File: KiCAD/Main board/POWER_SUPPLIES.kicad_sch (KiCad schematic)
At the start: 1 part, among them U18 12V

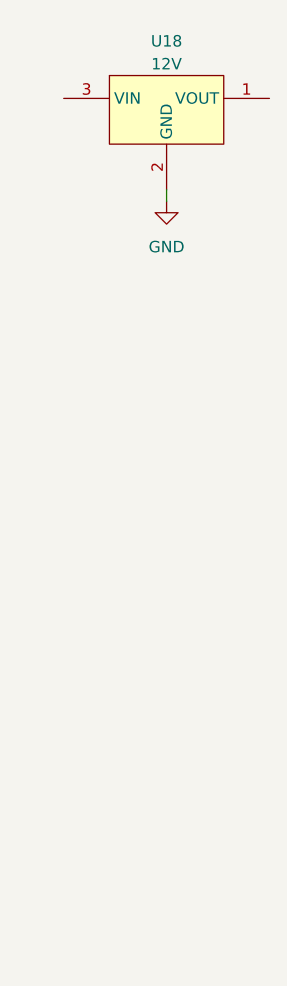
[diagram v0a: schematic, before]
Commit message: Worked on KiCAD
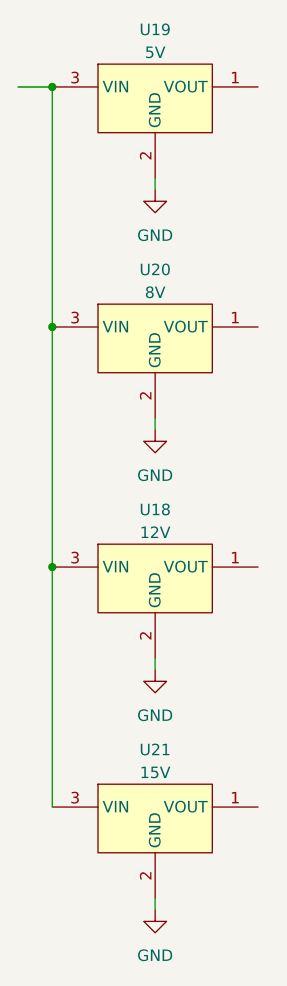
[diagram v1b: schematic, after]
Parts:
- added U19: 5V, Audio-DSP:BUCK_MAX17634C, symbol Audio_DSP:BUCK_5V_MAX17634C
- added U20: 8V, Audio-DSP:BUCK_MAX17634C, symbol Audio_DSP:BUCK_8V_MAX17634C
- added U21: 15V, Audio-DSP:BUCK_MAX17634C, symbol Audio_DSP:BUCK_15V_MAX17634C
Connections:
- net GND: now also U19.2 (GND), U20.2 (GND), U21.2 (GND)
- net at U18.3 (VIN): now also U19.3 (VIN), U20.3 (VIN), U21.3 (VIN)
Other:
- moved on the sheet: U18
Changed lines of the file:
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@@
 (kicad_sch (version 20230121) (generator eeschema)
   (paper "A4")
-  (wire (pts (xy 123.19 52.07) (xy 123.19 53.34))
-    (stroke (width 0) (type default))
-  )
-  (symbol (lib_id "power:GND") (at 123.19 53.34 0) (unit 1)
-    (in_bom yes) (on_board yes) (dnp no) (fields_autoplaced)
-    (property "Reference" "#PWR097" (at 123.19 59.69 0)
-      (effects (font (size 1.27 1.27)) hide)
-    )
-    (property "Value" "GND" (at 123.19 58.42 0)
-      (effects (font (size 1.27 1.27)))
-    )
-    (property "Footprint" "" (at 123.19 53.34 0)
-      (effects (font (size 1.27 1.27)) hide)
-    )
-    (property "Datasheet" "" (at 123.19 53.34 0)
+  (junction (at 110.49 93.98) (diameter 0) (color 0 0 0 0)
+  )
+  (junction (at 110.49 40.64) (diameter 0) (color 0 0 0 0)
+  )
+  (junction (at 110.49 67.31) (diameter 0) (color 0 0 0 0)
+  )
+  (wire (pts (xy 110.49 40.64) (xy 110.49 67.31))
+    (stroke (width 0) (type default))
+  )
+  (wire (pts (xy 121.92 77.47) (xy 121.92 78.74))
+    (stroke (width 0) (type default))
+  )
+  (wire (pts (xy 121.92 130.81) (xy 121.92 132.08))
+    (stroke (width 0) (type default))
+  )
+  (wire (pts (xy 110.49 67.31) (xy 110.49 93.98))
+    (stroke (width 0) (type default))
+  )
+  (wire (pts (xy 110.49 93.98) (xy 110.49 120.65))
+    (stroke (width 0) (type default))
+  )
+  (wire (pts (xy 121.92 104.14) (xy 121.92 105.41))
+    (stroke (width 0) (type default))
+  )
+  (wire (pts (xy 106.68 40.64) (xy 110.49 40.64))
+    (stroke (width 0) (type default))
+  )
+  (wire (pts (xy 121.92 50.8) (xy 121.92 52.07))
+    (stroke (width 0) (type default))
+  )
+  (symbol (lib_id "power:GND") (at 121.92 132.08 0) (unit 1)
+    (in_bom yes) (on_board yes) (dnp no) (fields_autoplaced)
+    (property "Reference" "#PWR098" (at 121.92 138.43 0)
+      (effects (font (size 1.27 1.27)) hide)
+    )
+    (property "Value" "GND" (at 121.92 137.16 0)
+      (effects (font (size 1.27 1.27)))
+    )
+    (property "Footprint" "" (at 121.92 132.08 0)
+      (effects (font (size 1.27 1.27)) hide)
+    )
+    (property "Datasheet" "" (at 121.92 132.08 0)
+      (effects (font (size 1.27 1.27)) hide)
+    )
+    (pin "1")
+    (instances
+      (project "Main board"
+        (path "/2f8cbac6-fd11-4240-8e40-3bb6952a0324/fc272ee1-9060-465b-85c1-b8364d68deb3"
+          (reference "#PWR098") (unit 1)
+        )
+      )
+    )
+  )
+  (symbol (lib_id "Audio_DSP:BUCK_5V_MAX17634C") (at 121.92 41.91 0) (unit 1)
+    (in_bom yes) (on_board yes) (dnp no) (fields_autoplaced)
+    (property "Reference" "U19" (at 121.92 34.29 0)
+      (effects (font (size 1.27 1.27)))
+    )
+    (property "Value" "5V" (at 121.92 36.83 0)
+      (effects (font (size 1.27 1.27)))
+    )
+    (property "Footprint" "Audio-DSP:BUCK_MAX17634C" (at 121.92 41.91 0)
+      (effects (font (size 1.27 1.27)) hide)
+    )
+    (property "Datasheet" "NA" (at 121.92 41.91 0)
+      (effects (font (size 1.27 1.27)) hide)
+    )
+    (pin "1")
+    (pin "2")
+    (pin "3")
+    (instances
+      (project "Main board"
+        (path "/2f8cbac6-fd11-4240-8e40-3bb6952a0324/fc272ee1-9060-465b-85c1-b8364d68deb3"
+          (reference "U19") (unit 1)
+        )
+      )
+    )
+  )
+  (symbol (lib_id "power:GND") (at 121.92 52.07 0) (unit 1)
+    (in_bom yes) (on_board yes) (dnp no) (fields_autoplaced)
+    (property "Reference" "#PWR0100" (at 121.92 58.42 0)
+      (effects (font (size 1.27 1.27)) hide)
+    )
+    (property "Value" "GND" (at 121.92 57.15 0)
+      (effects (font (size 1.27 1.27)))
+    )
+    (property "Footprint" "" (at 121.92 52.07 0)
+      (effects (font (size 1.27 1.27)) hide)
+    )
+    (property "Datasheet" "" (at 121.92 52.07 0)
+      (effects (font (size 1.27 1.27)) hide)
+    )
+    (pin "1")
+    (instances
+      (project "Main board"
+        (path "/2f8cbac6-fd11-4240-8e40-3bb6952a0324/fc272ee1-9060-465b-85c1-b8364d68deb3"
+          (reference "#PWR0100") (unit 1)
+        )
+      )
+    )
+  )
+  (symbol (lib_id "Audio_DSP:BUCK_8V_MAX17634C") (at 121.92 68.58 0) (unit 1)
+    (in_bom yes) (on_board yes) (dnp no) (fields_autoplaced)
+    (property "Reference" "U20" (at 121.92 60.96 0)
+      (effects (font (size 1.27 1.27)))
+    )
+    (property "Value" "8V" (at 121.92 63.5 0)
+      (effects (font (size 1.27 1.27)))
+    )
+    (property "Footprint" "Audio-DSP:BUCK_MAX17634C" (at 121.92 68.58 0)
+      (effects (font (size 1.27 1.27)) hide)
+    )
+    (property "Datasheet" "NA" (at 121.92 68.58 0)
+      (effects (font (size 1.27 1.27)) hide)
+    )
+    (pin "1")
+    (pin "2")
+    (pin "3")
+    (instances
+      (project "Main board"
+        (path "/2f8cbac6-fd11-4240-8e40-3bb6952a0324/fc272ee1-9060-465b-85c1-b8364d68deb3"
+          (reference "U20") (unit 1)
+        )
+      )
+    )
+  )
+  (symbol (lib_id "power:GND") (at 121.92 105.41 0) (unit 1)
+    (in_bom yes) (on_board yes) (dnp no) (fields_autoplaced)
+    (property "Reference" "#PWR097" (at 121.92 111.76 0)
+      (effects (font (size 1.27 1.27)) hide)
+    )
+    (property "Value" "GND" (at 121.92 110.49 0)
+      (effects (font (size 1.27 1.27)))
+    )
+    (property "Footprint" "" (at 121.92 105.41 0)
+      (effects (font (size 1.27 1.27)) hide)
+    )
+    (property "Datasheet" "" (at 121.92 105.41 0)
       (effects (font (size 1.27 1.27)) hide)
     )
@@
     )
   )
-  (symbol (lib_id "Audio_DSP:BUCK_12V_MAX17634C") (at 123.19 43.18 0) (unit 1)
-    (in_bom yes) (on_board yes) (dnp no) (fields_autoplaced)
-    (property "Reference" "U18" (at 123.19 35.56 0)
-      (effects (font (size 1.27 1.27)))
-    )
-    (property "Value" "12V" (at 123.19 38.1 0)
-      (effects (font (size 1.27 1.27)))
-    )
-    (property "Footprint" "Audio-DSP:BUCK_MAX17634C" (at 123.19 43.18 0)
-      (effects (font (size 1.27 1.27)) hide)
-    )
-    (property "Datasheet" "NA" (at 123.19 43.18 0)
+  (symbol (lib_id "Audio_DSP:BUCK_12V_MAX17634C") (at 121.92 95.25 0) (unit 1)
+    (in_bom yes) (on_board yes) (dnp no) (fields_autoplaced)
+    (property "Reference" "U18" (at 121.92 87.63 0)
+      (effects (font (size 1.27 1.27)))
+    )
+    (property "Value" "12V" (at 121.92 90.17 0)
+      (effects (font (size 1.27 1.27)))
+    )
+    (property "Footprint" "Audio-DSP:BUCK_MAX17634C" (at 121.92 95.25 0)
+      (effects (font (size 1.27 1.27)) hide)
+    )
+    (property "Datasheet" "NA" (at 121.92 95.25 0)
       (effects (font (size 1.27 1.27)) hide)
     )
@@
         )
       )
+    )
+  )
+  (symbol (lib_id "Audio_DSP:BUCK_15V_MAX17634C") (at 121.92 121.92 0) (unit 1)
+    (in_bom yes) (on_board yes) (dnp no) (fields_autoplaced)
+    (property "Reference" "U21" (at 121.92 114.3 0)
+      (effects (font (size 1.27 1.27)))
+    )
+    (property "Value" "15V" (at 121.92 116.84 0)
+      (effects (font (size 1.27 1.27)))
+    )
+    (property "Footprint" "Audio-DSP:BUCK_MAX17634C" (at 121.92 121.92 0)
+      (effects (font (size 1.27 1.27)) hide)
+    )
+    (property "Datasheet" "NA" (at 121.92 121.92 0)
+      (effects (font (size 1.27 1.27)) hide)
+    )
+    (pin "1")
+    (pin "2")
+    (pin "3")
+    (instances
+      (project "Main board"
+        (path "/2f8cbac6-fd11-4240-8e40-3bb6952a0324/fc272ee1-9060-465b-85c1-b8364d68deb3"
+          (reference "U21") (unit 1)
+        )
+      )
+    )
+  )
+  (symbol (lib_id "power:GND") (at 121.92 78.74 0) (unit 1)
+    (in_bom yes) (on_board yes) (dnp no) (fields_autoplaced)
+    (property "Reference" "#PWR099" (at 121.92 85.09 0)
+      (effects (font (size 1.27 1.27)) hide)
+    )
+    (property "Value" "GND" (at 121.92 83.82 0)
+      (effects (font (size 1.27 1.27)))
+    )
+    (property "Footprint" "" (at 121.92 78.74 0)
+      (effects (font (size 1.27 1.27)) hide)
+    )
+    (property "Datasheet" "" (at 121.92 78.74 0)
+      (effects (font (size 1.27 1.27)) hide)
+    )
+    (pin "1")
+    (instances
+      (project "Main board"
+        (path "/2f8cbac6-fd11-4240-8e40-3bb6952a0324/fc272ee1-9060-465b-85c1-b8364d68deb3"
+          (reference "#PWR099") (unit 1)
+        )
+      )
